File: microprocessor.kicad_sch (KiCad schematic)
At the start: 45 parts, among them J15 Conn_01x03, J4 Conn_02x03_Odd_Even, U3 ATxmega256A3U-AU, X1 ABLS-16.000MHZ-B4-T

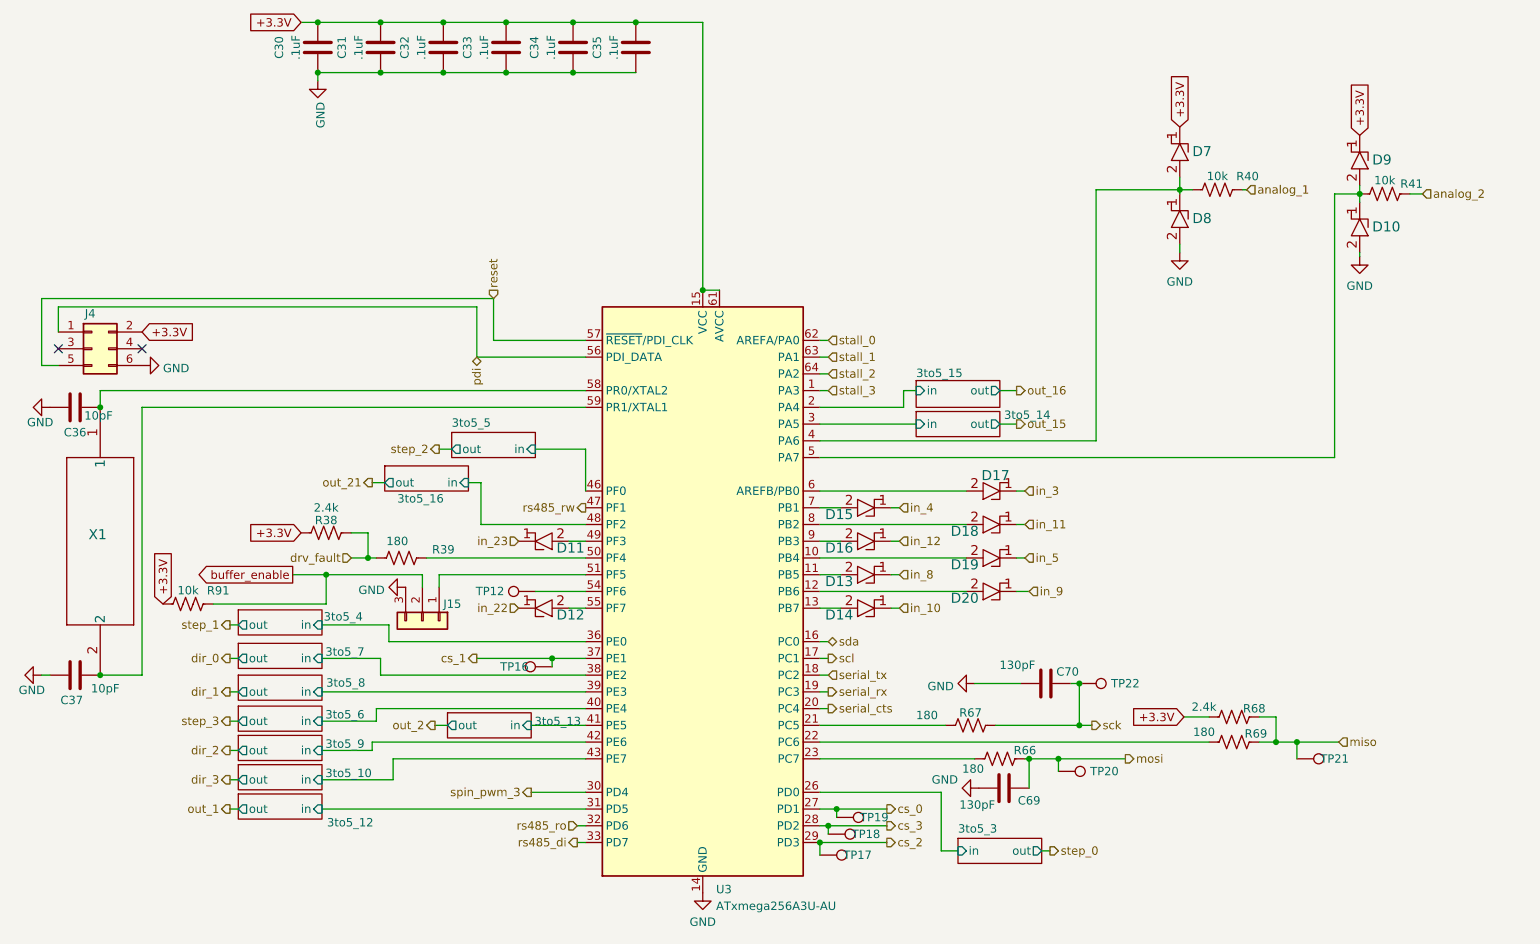
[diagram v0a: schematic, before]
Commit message: All DRC errors cleared after conversion to Kicad V7
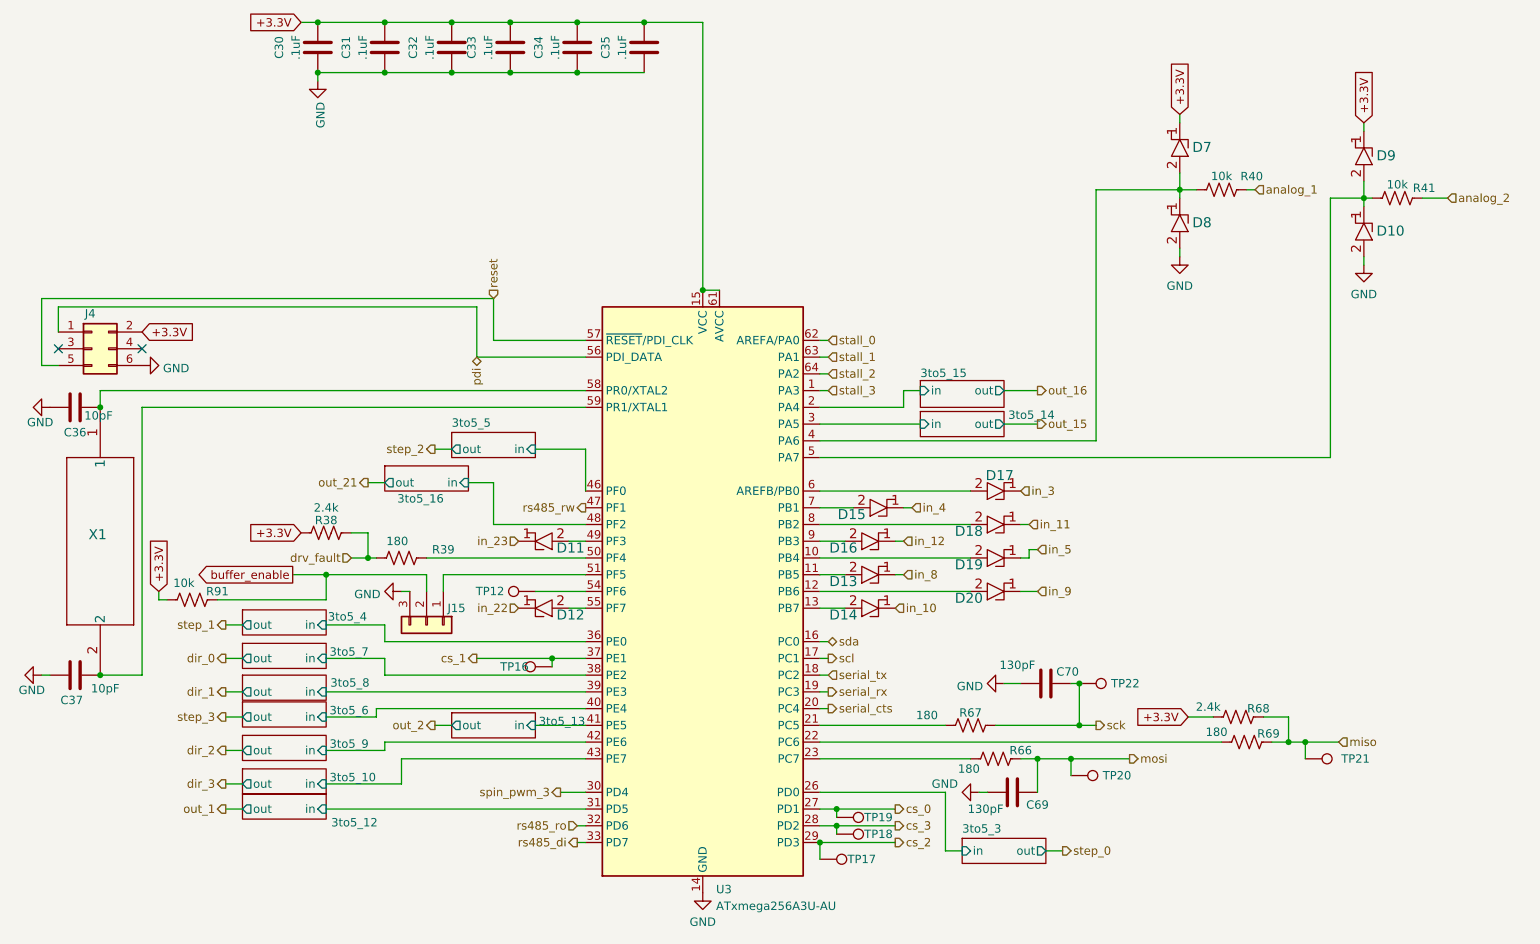
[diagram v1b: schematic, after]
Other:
- moved on the sheet: C31, C32, C33, C34, C35, C69, D10, D13, D14, D15, D16, D17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

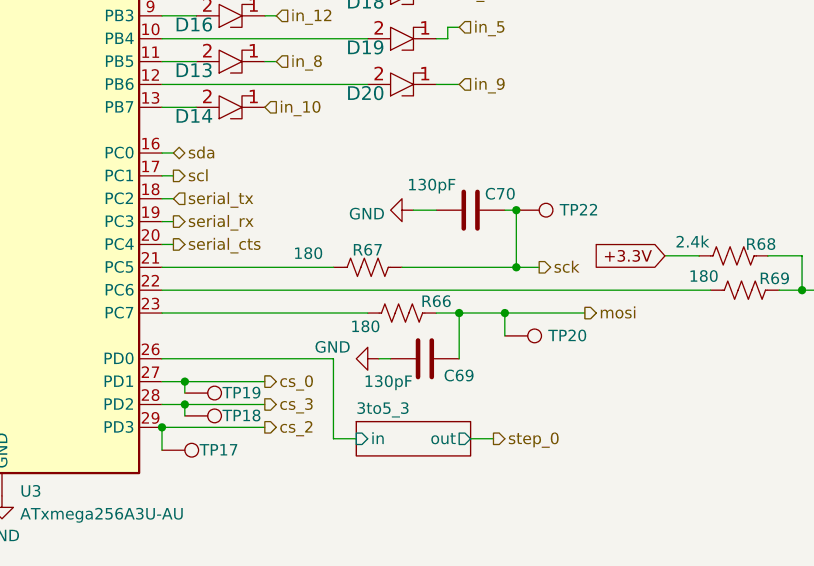
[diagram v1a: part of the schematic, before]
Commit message: swapped avr pins 21 and 23 (mosi and sck) to accomodate xmegaa3 chip
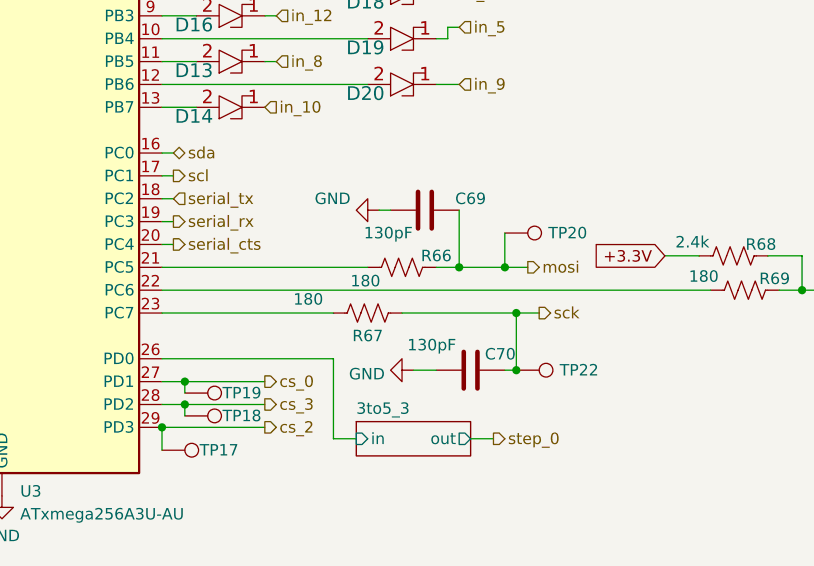
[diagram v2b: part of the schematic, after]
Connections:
- net at R67.1: now also U3.23 (PC7); no longer U3.21 (PC5)
- net at R66.1: now also U3.21 (PC5); no longer U3.23 (PC7)
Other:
- moved on the sheet: C69, C70, R66, R67, TP20, TP22
